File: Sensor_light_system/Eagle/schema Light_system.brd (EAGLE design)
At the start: 60 x 50 mm, 23 parts, among them IC1 STM32F030C8T6TR, J1 12_WAY_CON

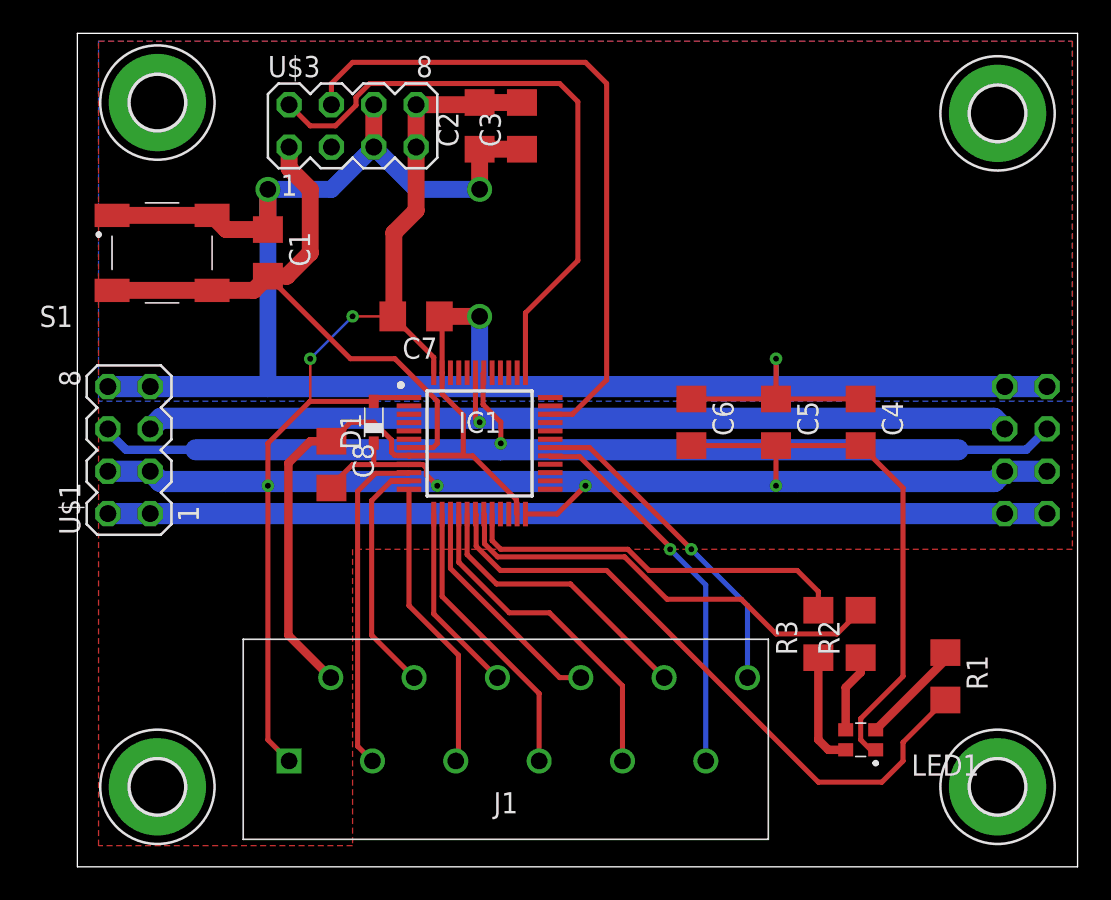
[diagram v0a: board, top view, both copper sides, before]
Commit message: eagle
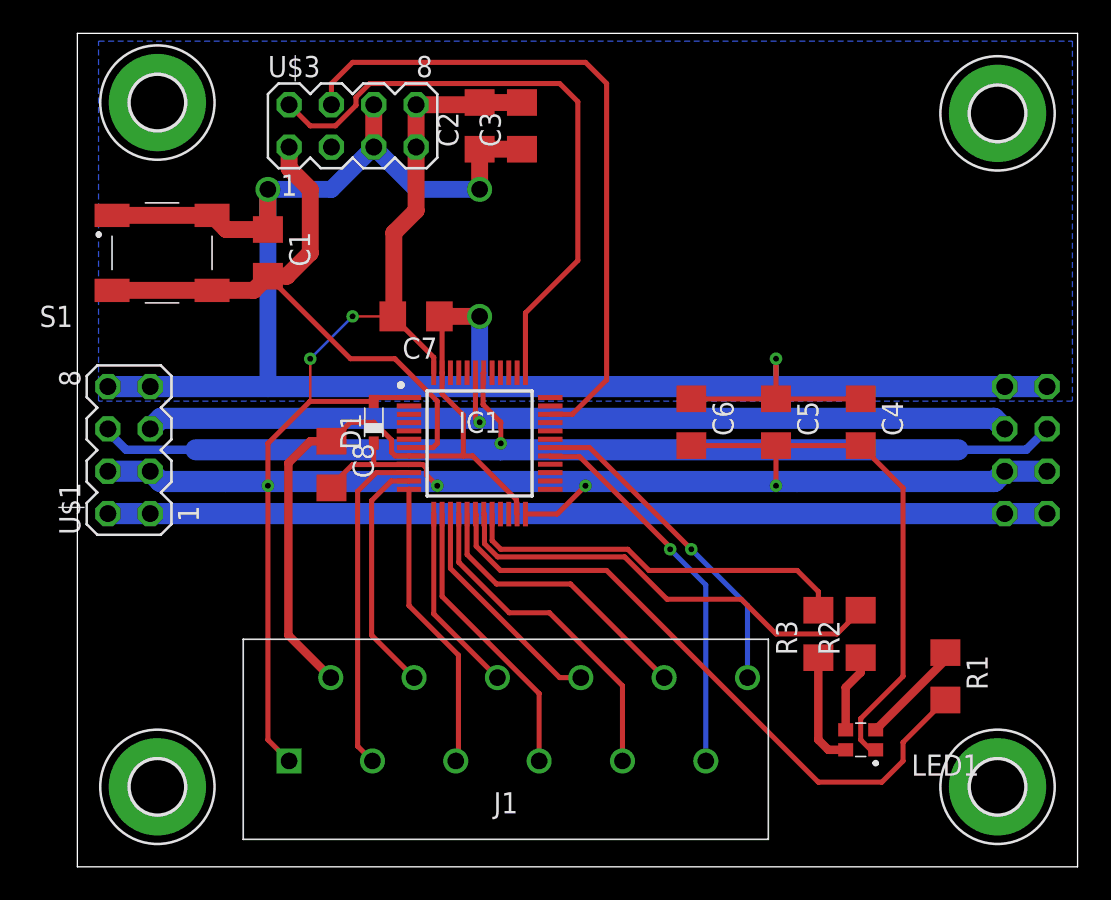
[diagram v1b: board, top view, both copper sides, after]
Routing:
- net GND: track 167.5 -> 164.2 mm
- net PA1: track 15.5 -> 14.4 mm
- removed copper zone on layer 1, net GND
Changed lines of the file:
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@@
 <via x="41.91" y="22.86" extent="1-16" drill="0.35"/>
 <wire x1="41.91" y1="25.27" x2="41.91" y2="22.86" width="0.3048" layer="1"/>
-<wire x1="46.99" y1="25.27" x2="46.86" y2="25.27" width="0.3048" layer="1"/>
 <wire x1="41.91" y1="22.86" x2="42.164" y2="23.114" width="0.3048" layer="16"/>
 <wire x1="42.164" y1="23.114" x2="43.18" y2="23.114" width="0.3048" layer="16"/>
@@
 <wire x1="49.53" y1="11.43" x2="49.53" y2="22.73" width="0.3048" layer="1"/>
 <wire x1="36.83" y1="25.27" x2="41.91" y2="25.27" width="0.3048" layer="1"/>
-<wire x1="41.91" y1="25.27" x2="46.99" y2="25.27" width="0.3048" layer="1"/>
 <via x="30.48" y="22.86" extent="1-16" drill="0.35"/>
 <wire x1="30.48" y1="22.86" x2="30.48" y2="23.114" width="0.3048" layer="16"/>
@@
 <wire x1="13.97" y1="27.94" x2="13.95" y2="27.92" width="0.1524" layer="1"/>
 <wire x1="13.97" y1="30.48" x2="16.51" y2="33.02" width="0.1524" layer="16"/>
+<wire x1="41.91" y1="25.27" x2="46.99" y2="25.27" width="0.3048" layer="1"/>
 </signal>
 <signal name="GND">
@@
 <wire x1="15.24" y1="25.53" x2="16.38" y2="26.67" width="0.3048" layer="1"/>
 <wire x1="16.38" y1="26.67" x2="17.78" y2="26.67" width="0.3048" layer="1"/>
-<wire x1="18.8497" y1="24.87375" x2="19.02825" y2="24.6952" width="0.3048" layer="1"/>
-<wire x1="19.02825" y1="24.6952" x2="19.8468" y2="24.6952" width="0.3048" layer="1"/>
-<wire x1="19.8468" y1="24.6952" x2="19.892" y2="24.65" width="0.3048" layer="1"/>
 <wire x1="17.78" y1="26.67" x2="18.8497" y2="25.6003" width="0.3048" layer="1"/>
-<wire x1="18.8497" y1="25.6003" x2="18.8497" y2="24.87375" width="0.3048" layer="1"/>
+<wire x1="18.8497" y1="25.6003" x2="18.8497" y2="25.4" width="0.3048" layer="1"/>
 <via x="41.91" y="30.48" extent="1-16" drill="0.35"/>
+<wire x1="18.8497" y1="25.4" x2="18.8497" y2="24.87375" width="0.3048" layer="1"/>
 <wire x1="41.91" y1="28.07" x2="41.91" y2="30.48" width="0.3048" layer="1"/>
 <wire x1="41.91" y1="28.81" x2="41.91" y2="30.48" width="0.3048" layer="16"/>
 <wire x1="36.83" y1="28.07" x2="41.91" y2="28.07" width="0.3048" layer="1"/>
 <wire x1="41.91" y1="28.07" x2="46.99" y2="28.07" width="0.3048" layer="1"/>
-<wire x1="19.892" y1="24.65" x2="19.9372" y2="24.6952" width="0.3048" layer="1"/>
-<wire x1="19.9372" y1="24.6952" x2="23.15" y2="24.6952" width="0.3048" layer="1"/>
 <wire x1="23.15" y1="27.098" x2="21.88" y2="28.368" width="0.3048" layer="1"/>
 <wire x1="21.88" y1="28.368" x2="21.88" y2="29.638" width="0.3048" layer="1"/>
@@
 <wire x1="26.38" y1="21.162" x2="26.3348" y2="21.2072" width="0.3048" layer="1"/>
 <wire x1="26.3348" y1="21.2072" x2="26.3348" y2="22.02575" width="0.3048" layer="1"/>
-<wire x1="26.3348" y1="22.02575" x2="23.71055" y2="24.65" width="0.3048" layer="1"/>
-<wire x1="23.71055" y1="24.65" x2="19.892" y2="24.65" width="0.3048" layer="1"/>
+<wire x1="23.71055" y1="24.65" x2="26.3348" y2="22.02575" width="0.3048" layer="1"/>
 <via x="11.43" y="40.64" extent="1-16" drill="1"/>
 <wire x1="11.43" y1="40.64" x2="11.43" y2="38.23" width="1.016" layer="1"/>
@@
 <vertex x="1.27" y="27.94"/>
 </polygon>
-<polygon width="0.1524" layer="1">
-<vertex x="1.27" y="49.53"/>
-<vertex x="59.69" y="49.53"/>
-<vertex x="59.69" y="19.05"/>
-<vertex x="16.51" y="19.05"/>
-<vertex x="16.51" y="1.27"/>
-<vertex x="1.27" y="1.27"/>
-</polygon>
+<wire x1="19.07345" y1="24.65" x2="19.892" y2="24.65" width="0.3048" layer="1"/>
+<wire x1="18.8497" y1="24.87375" x2="19.07345" y2="24.65" width="0.3048" layer="1"/>
+<wire x1="23.15" y1="24.6952" x2="23.1048" y2="24.65" width="0.3048" layer="1"/>
+<wire x1="23.15" y1="24.6952" x2="23.1952" y2="24.65" width="0.3048" layer="1"/>
+<wire x1="23.1952" y1="24.65" x2="23.71055" y2="24.65" width="0.3048" layer="1"/>
+<wire x1="23.1048" y1="24.65" x2="19.892" y2="24.65" width="0.3048" layer="1"/>
 </signal>
 <signal name="PA0">
 <contactref element="IC1" pad="10"/>
 <contactref element="J1" pad="3"/>
-<wire x1="17.88525" y1="23.6048" x2="19.8468" y2="23.6048" width="0.3048" layer="1"/>
-<wire x1="19.8468" y1="23.6048" x2="19.892" y2="23.65" width="0.3048" layer="1"/>
-<wire x1="16.811" y1="22.53055" x2="16.811" y2="7.239" width="0.3048" layer="1"/>
+<wire x1="16.811" y1="7.239" x2="16.811" y2="22.53055" width="0.3048" layer="1"/>
 <wire x1="17.7" y1="6.35" x2="16.811" y2="7.239" width="0.3048" layer="1"/>
-<wire x1="17.88525" y1="23.6048" x2="16.811" y2="22.53055" width="0.3048" layer="1"/>
+<wire x1="16.811" y1="22.53055" x2="17.93045" y2="23.65" width="0.3048" layer="1"/>
+<wire x1="17.93045" y1="23.65" x2="19.892" y2="23.65" width="0.3048" layer="1"/>
 </signal>
 <signal name="PA1">
@@
 <contactref element="J1" pad="4"/>
 <wire x1="20.2" y1="11.35" x2="17.653" y2="13.897" width="0.3048" layer="1"/>
-<wire x1="17.653" y1="13.897" x2="17.653" y2="21.971" width="0.3048" layer="1"/>
+<wire x1="17.653" y1="13.897" x2="17.653" y2="21.59" width="0.3048" layer="1"/>
+<wire x1="18.8296" y1="23.1476" x2="19.8896" y2="23.1476" width="0.3048" layer="1"/>
+<wire x1="19.8896" y1="23.1476" x2="19.892" y2="23.15" width="0.3048" layer="1"/>
+<wire x1="17.653" y1="21.59" x2="17.653" y2="21.971" width="0.3048" layer="1"/>
 <wire x1="17.653" y1="21.971" x2="18.8296" y2="23.1476" width="0.3048" layer="1"/>
-<wire x1="18.8296" y1="23.1476" x2="19.892" y2="23.1476" width="0.3048" layer="1"/>
-<wire x1="19.892" y1="23.15" x2="18.832" y2="23.15" width="0.3048" layer="1"/>
-<wire x1="18.832" y1="23.15" x2="18.8296" y2="23.1476" width="0.3048" layer="1"/>
 </signal>
 <signal name="PA2">
